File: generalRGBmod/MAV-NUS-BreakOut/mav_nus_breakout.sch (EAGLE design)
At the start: 24 parts

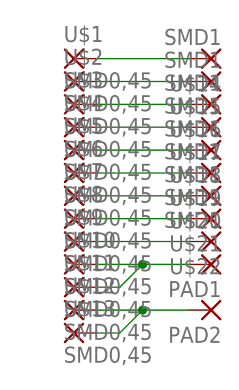
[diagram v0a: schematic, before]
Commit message: initial commit DIY projects
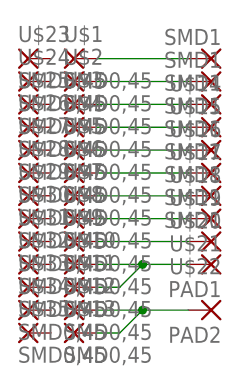
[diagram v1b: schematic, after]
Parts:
- added U$23, U$24, U$25, U$26, U$27, U$28, U$29, U$30, U$31, U$32, U$33, U$34, U$35: SMD0,45, wirepad:SMD0,45
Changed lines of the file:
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@@
 <?xml version="1.0" encoding="utf-8"?>
 <!DOCTYPE eagle SYSTEM "eagle.dtd">
-<eagle version="7.6.0">
+<eagle version="7.7.0">
 <drawing>
 <settings>
@@
 <part name="U$12" library="wirepad" deviceset="SMD0,45" device=""/>
 <part name="U$13" library="wirepad" deviceset="SMD0,45" device=""/>
+<part name="U$23" library="wirepad" deviceset="SMD0,45" device=""/>
+<part name="U$24" library="wirepad" deviceset="SMD0,45" device=""/>
+<part name="U$25" library="wirepad" deviceset="SMD0,45" device=""/>
+<part name="U$26" library="wirepad" deviceset="SMD0,45" device=""/>
+<part name="U$27" library="wirepad" deviceset="SMD0,45" device=""/>
+<part name="U$28" library="wirepad" deviceset="SMD0,45" device=""/>
+<part name="U$29" library="wirepad" deviceset="SMD0,45" device=""/>
+<part name="U$30" library="wirepad" deviceset="SMD0,45" device=""/>
+<part name="U$31" library="wirepad" deviceset="SMD0,45" device=""/>
+<part name="U$32" library="wirepad" deviceset="SMD0,45" device=""/>
+<part name="U$33" library="wirepad" deviceset="SMD0,45" device=""/>
+<part name="U$34" library="wirepad" deviceset="SMD0,45" device=""/>
+<part name="U$35" library="wirepad" deviceset="SMD0,45" device=""/>
 </parts>
 <sheets>
@@
 <instance part="U$12" gate="G$1" x="2.54" y="12.7"/>
 <instance part="U$13" gate="G$1" x="2.54" y="10.16"/>
+<instance part="U$23" gate="G$1" x="-2.54" y="40.64"/>
+<instance part="U$24" gate="G$1" x="-2.54" y="38.1"/>
+<instance part="U$25" gate="G$1" x="-2.54" y="35.56"/>
+<instance part="U$26" gate="G$1" x="-2.54" y="33.02"/>
+<instance part="U$27" gate="G$1" x="-2.54" y="30.48"/>
+<instance part="U$28" gate="G$1" x="-2.54" y="27.94"/>
+<instance part="U$29" gate="G$1" x="-2.54" y="25.4"/>
+<instance part="U$30" gate="G$1" x="-2.54" y="22.86"/>
+<instance part="U$31" gate="G$1" x="-2.54" y="20.32"/>
+<instance part="U$32" gate="G$1" x="-2.54" y="17.78"/>
+<instance part="U$33" gate="G$1" x="-2.54" y="15.24"/>
+<instance part="U$34" gate="G$1" x="-2.54" y="12.7"/>
+<instance part="U$35" gate="G$1" x="-2.54" y="10.16"/>
 </instances>
 <busses>
